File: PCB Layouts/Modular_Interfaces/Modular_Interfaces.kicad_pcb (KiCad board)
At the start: 2 copper layers, 92.8 x 84.5 mm, 37 parts, among them J1 Conn_01x03_Socket, J1 Conn_01x04_Socket, J1 RJ45_LED, J1 USB_A, J2 Conn_01x10_Socket, J3 Conn_01x10_Socket, U4 ENC28J60x-SS, Y1 25MHz

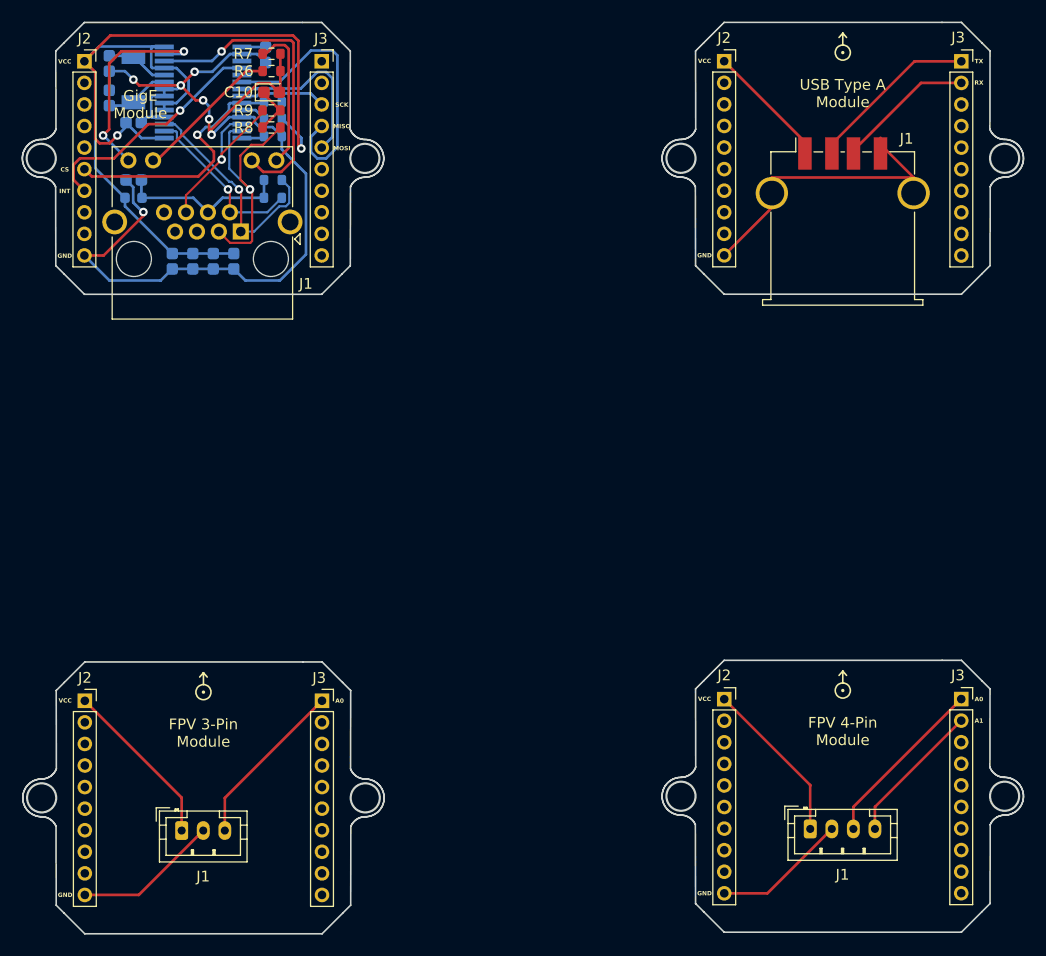
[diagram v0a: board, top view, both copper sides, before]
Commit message: Updating gerber files of the unified design
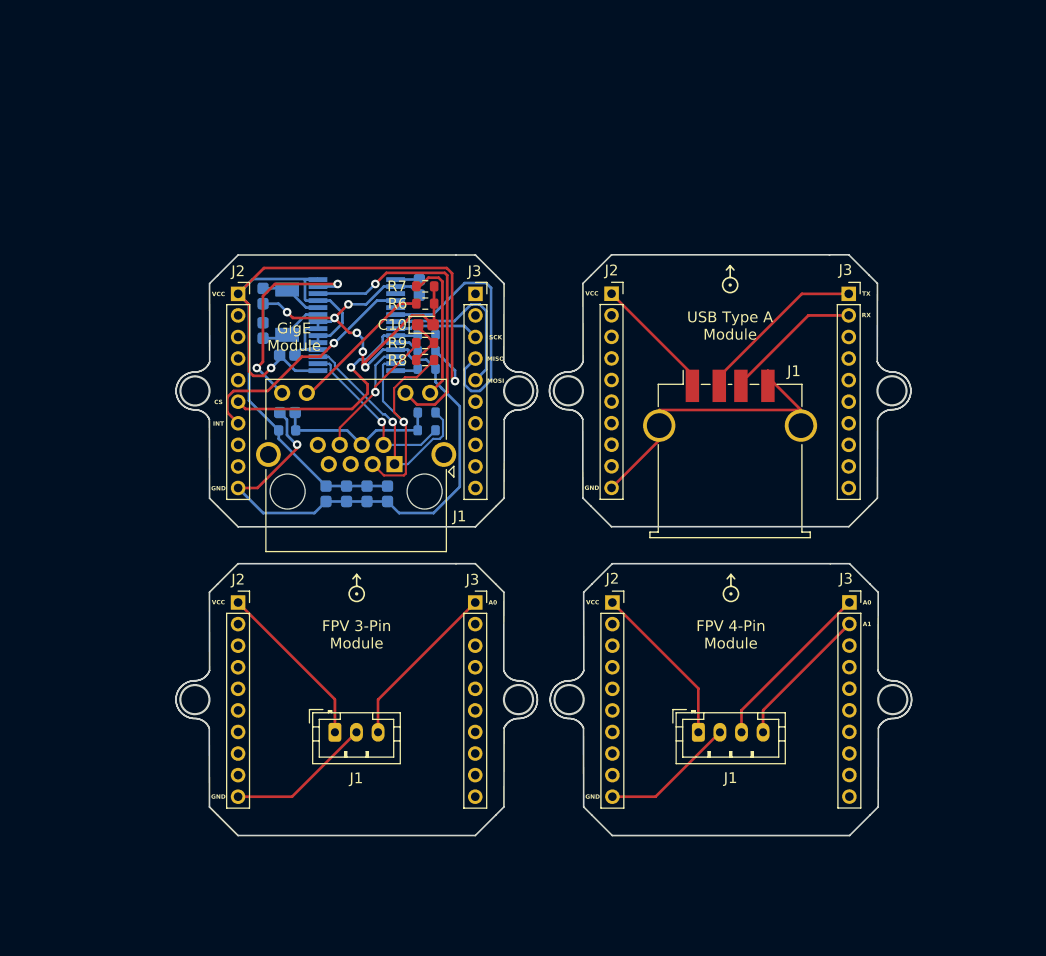
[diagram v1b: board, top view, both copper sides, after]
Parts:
- moved C4 25.8 mm to (131.3, 74.0)
- moved R5 25.8 mm to (144.2, 81.0)
- moved C10 25.8 mm to (144.1, 71.2)
- moved J3 25.8 mm to (148.7, 68.3)
- moved R2 25.8 mm to (144.2, 73.6)
- moved C2 25.8 mm to (129.1, 71.7)
- moved C3 25.8 mm to (129.1, 68.5)
- moved J1 25.8 mm to (141.2, 84.1)
- moved J2 25.8 mm to (126.7, 68.3)
- moved C5 25.8 mm to (134.9, 86.9)
- moved C6 25.8 mm to (136.8, 86.9)
- moved L1 25.8 mm to (131.3, 81.0)
- moved R1 25.8 mm to (144.2, 72.1)
- moved R3 25.8 mm to (144.2, 75.3)
- moved R8 25.8 mm to (144.1, 74.5)
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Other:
- board size 92.8 x 84.5 mm -> 68.2 x 53.8 mm
- board text removed: "ANT"
- board text removed: "BAT"
- board text removed: "BTN"
- board text removed: "Bitcraze"
- board text removed: "Crazyflie 2.0"
- board text removed: "M1"
- board text removed: "M2"
- board text removed: "M3"
- board text removed: "M4"
- board text removed: "SWD BOTTOM"
- board text removed: "uUSB TOP"
